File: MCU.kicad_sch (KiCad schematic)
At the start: 20 parts, among them U2 STM32L476RGTx, Y2 Crystal

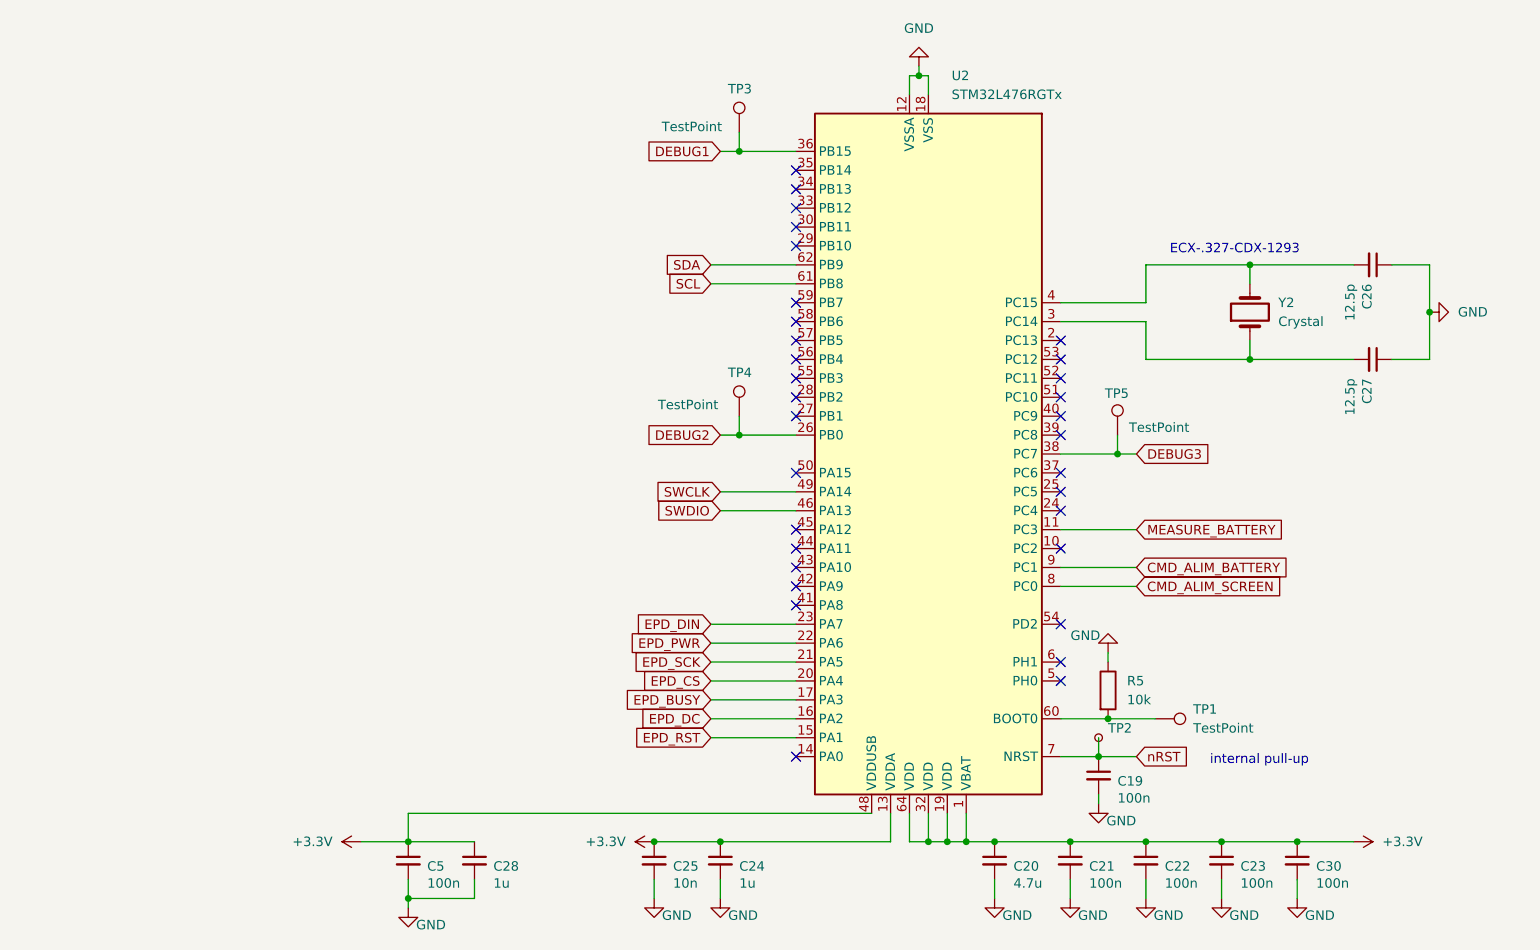
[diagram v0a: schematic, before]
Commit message: schema v1
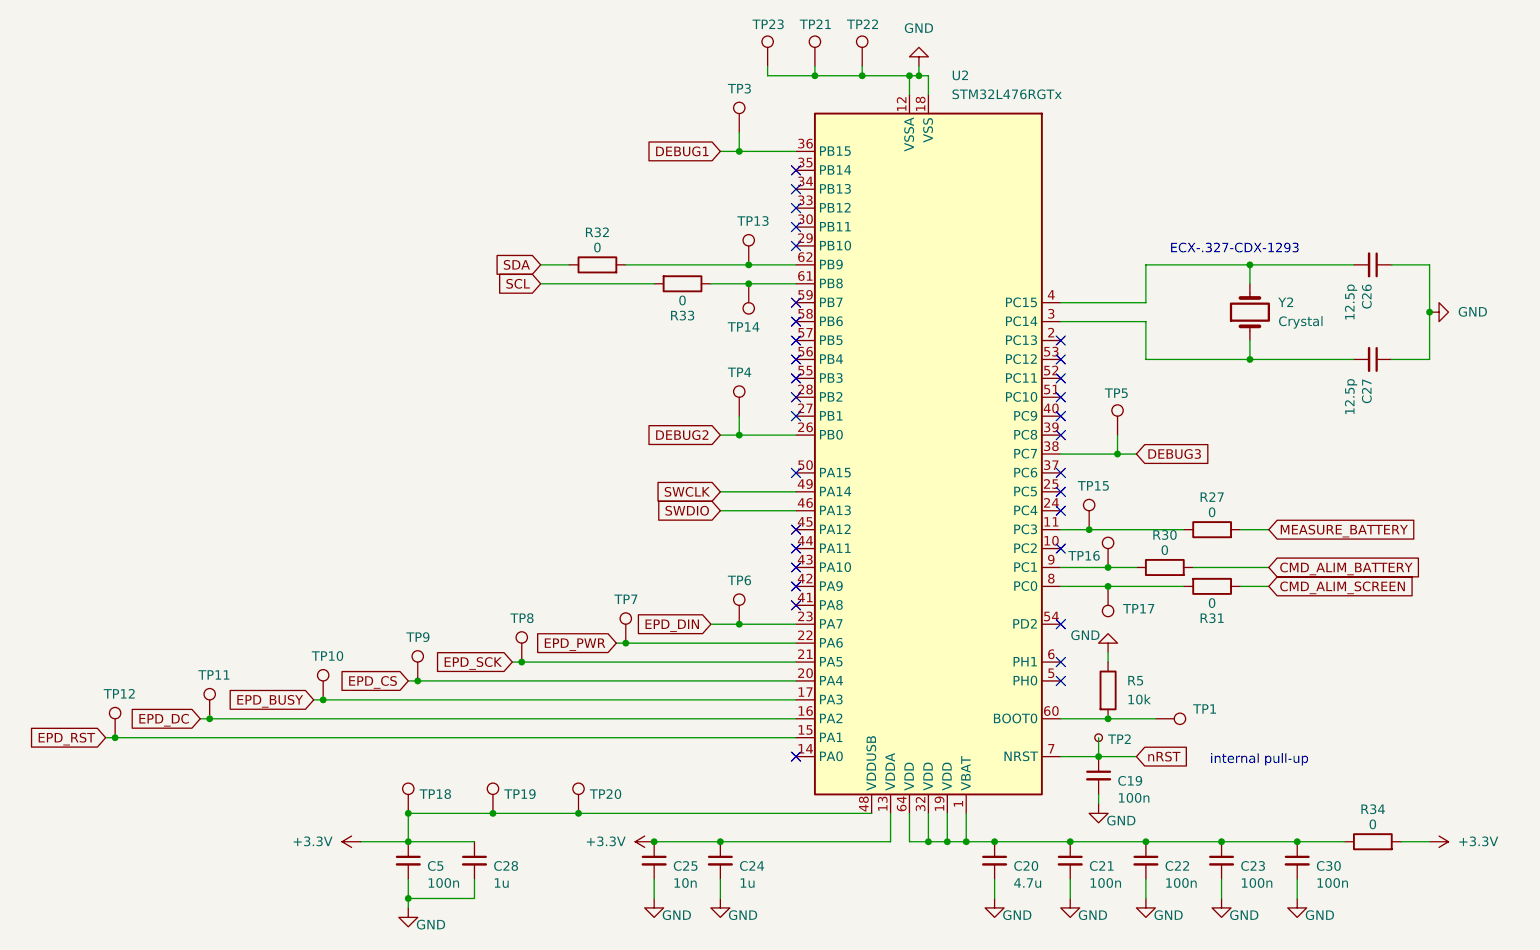
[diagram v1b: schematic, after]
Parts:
- added R27, R30, R31, R32, R33, R34: 0, symbol Device:R
- added TP10, TP11, TP12, TP13, TP14, TP15, TP16, TP17, TP18, TP19, TP20, TP21, TP22, TP23, TP6, TP7, TP8, TP9: TestPoint, symbol Connector:TestPoint
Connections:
- net +3.3V: now also R34.2, TP18.1, TP19.1, TP20.1; no longer C20.1, C21.1, C22.1, C23.1, C30.1, U2.1 (VBAT), U2.19 (VDD), U2.32 (VDD), U2.64 (VDD)
- net CMD_ALIM_BATTERY: now also R30.2; no longer U2.9 (PC1)
- net CMD_ALIM_SCREEN: now also R31.1; no longer U2.8 (PC0)
- net EPD_BUSY: now also TP10.1
- net EPD_CS: now also TP9.1
- net EPD_DC: now also TP11.1
- net EPD_DIN: now also TP6.1
- net EPD_PWR: now also TP7.1
- net EPD_RST: now also TP12.1
- net EPD_SCK: now also TP8.1
- net GND: now also TP21.1, TP22.1, TP23.1
- net MEASURE_BATTERY: now also R27.2; no longer U2.11 (PC3)
- net SCL: now also R33.2; no longer U2.61 (PB8)
- net SDA: now also R32.1; no longer U2.62 (PB9)
- new net: R32.2, TP13.1, U2.62 (PB9)
- new net: R30.1, TP16.1, U2.9 (PC1)
- new net: C20.1, C21.1, C22.1, C23.1, C30.1, R34.1, U2.1 (VBAT), U2.19 (VDD), U2.32 (VDD), U2.64 (VDD)
- new net: R27.1, TP15.1, U2.11 (PC3)
- new net: R33.1, TP14.1, U2.61 (PB8)
- new net: R31.2, TP17.1, U2.8 (PC0)

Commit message: Connecteurs + sourcing
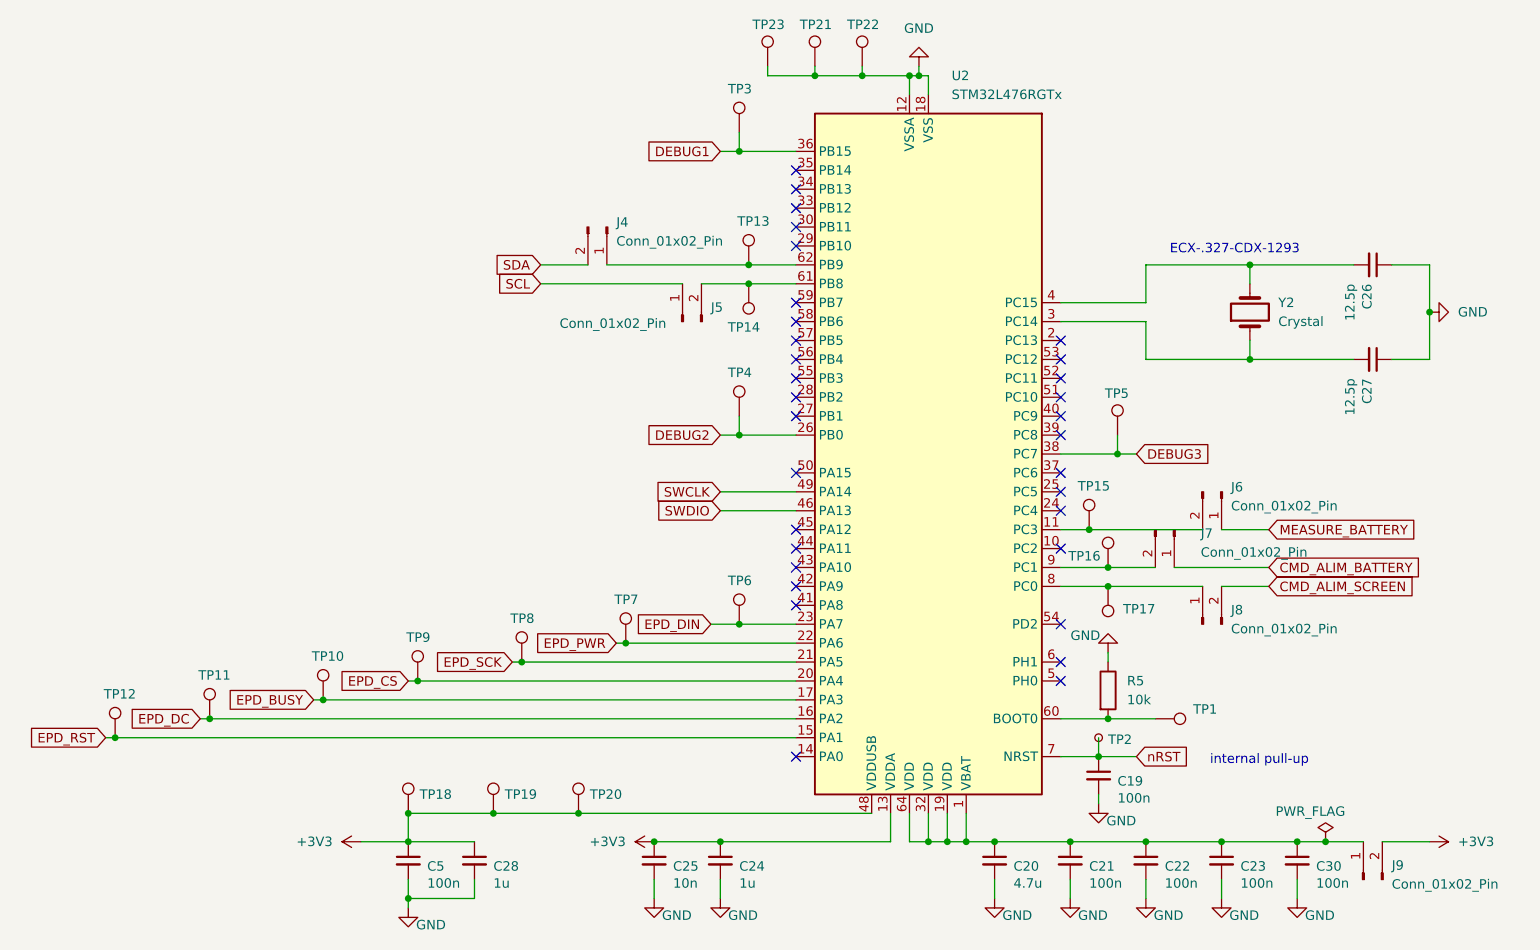
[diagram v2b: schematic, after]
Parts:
- removed R27, R30, R31, R32, R33, R34: 0, symbol Device:R
- added J4, J6, J7: Conn_01x02_Pin, Connector_PinHeader_2.54mm:PinHeader_1x02_P2.54mm_Vertical_SMD_Pin1Right, symbol Connector:Conn_01x02_Pin
- added J5, J8, J9: Conn_01x02_Pin, Connector_PinHeader_2.54mm:PinHeader_1x02_P2.54mm_Vertical_SMD_Pin1Left, symbol Connector:Conn_01x02_Pin
- C19: footprint (none) -> Capacitor_SMD:C_0402_1005Metric
- C20: footprint (none) -> Capacitor_SMD:C_0805_2012Metric
- C21, C22, C23, C30, C5: footprint (none) -> Capacitor_SMD:C_0402_1005Metric; LCSC (none) -> C1525
- C24, C28: footprint (none) -> Capacitor_SMD:C_0603_1608Metric; LCSC (none) -> C15849
- C25: footprint (none) -> Capacitor_SMD:C_0603_1608Metric; LCSC (none) -> C57112
- C26, C27: footprint (none) -> Capacitor_SMD:C_0402_1005Metric; LCSC (none) -> C1547
- R5: footprint (none) -> Resistor_SMD:R_0603_1608Metric
- TP1, TP10, TP11, TP12, TP13, TP14, TP15, TP16, TP17, TP18, TP19, TP2, TP20, TP21, TP22, TP23, TP3, TP4, TP5, TP6, TP7, TP8, TP9: footprint (none) -> TestPoint:TestPoint_Pad_D1.5mm
- Y2: footprint (none) -> Crystal:Crystal_SMD_3215-2Pin_3.2x1.5mm
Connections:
- net CMD_ALIM_BATTERY: now also J7.1 (Pin_1)
- net CMD_ALIM_SCREEN: now also J8.2 (Pin_2)
- net MEASURE_BATTERY: now also J6.1 (Pin_1)
- net SCL: now also J5.1 (Pin_1)
- net SDA: now also J4.2 (Pin_2)
- net at TP13.1, U2.62 (PB9): now also J4.1 (Pin_1)
- net at TP16.1, U2.9 (PC1): now also J7.2 (Pin_2)
- net at C20.1, C21.1, C22.1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: now also J9.1 (Pin_1)
- net at TP15.1, U2.11 (PC3): now also J6.2 (Pin_2)
- net at TP14.1, U2.61 (PB8): now also J5.2 (Pin_2)
- net at TP17.1, U2.8 (PC0): now also J8.1 (Pin_1)
- net +3.3V renamed +3V3
- net +3V3: now also J9.2 (Pin_2)
